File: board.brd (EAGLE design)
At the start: 25.3 x 23.8 mm, 30 parts, among them U3 ATTINY1607-MFR, U4 RV-8803, X2 JST_SM02B-SRSS-TB

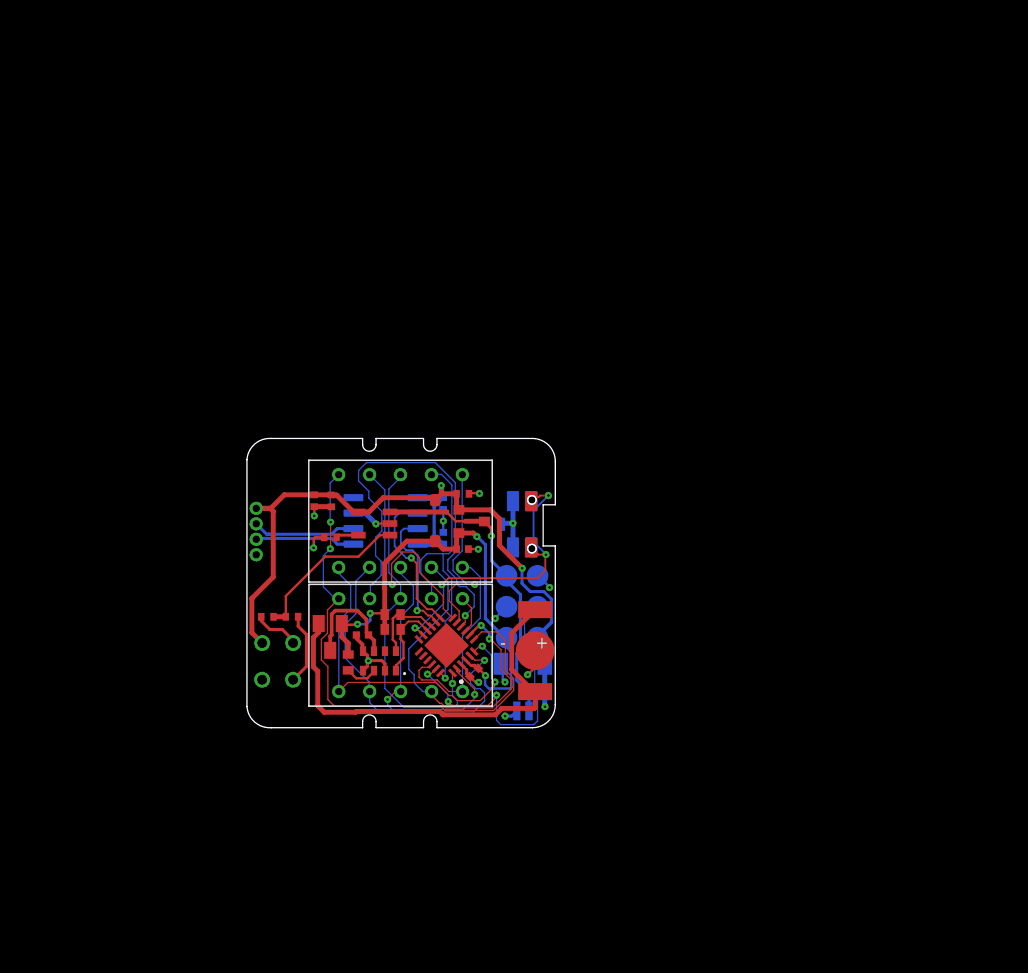
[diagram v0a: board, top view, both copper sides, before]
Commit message: added next dev board
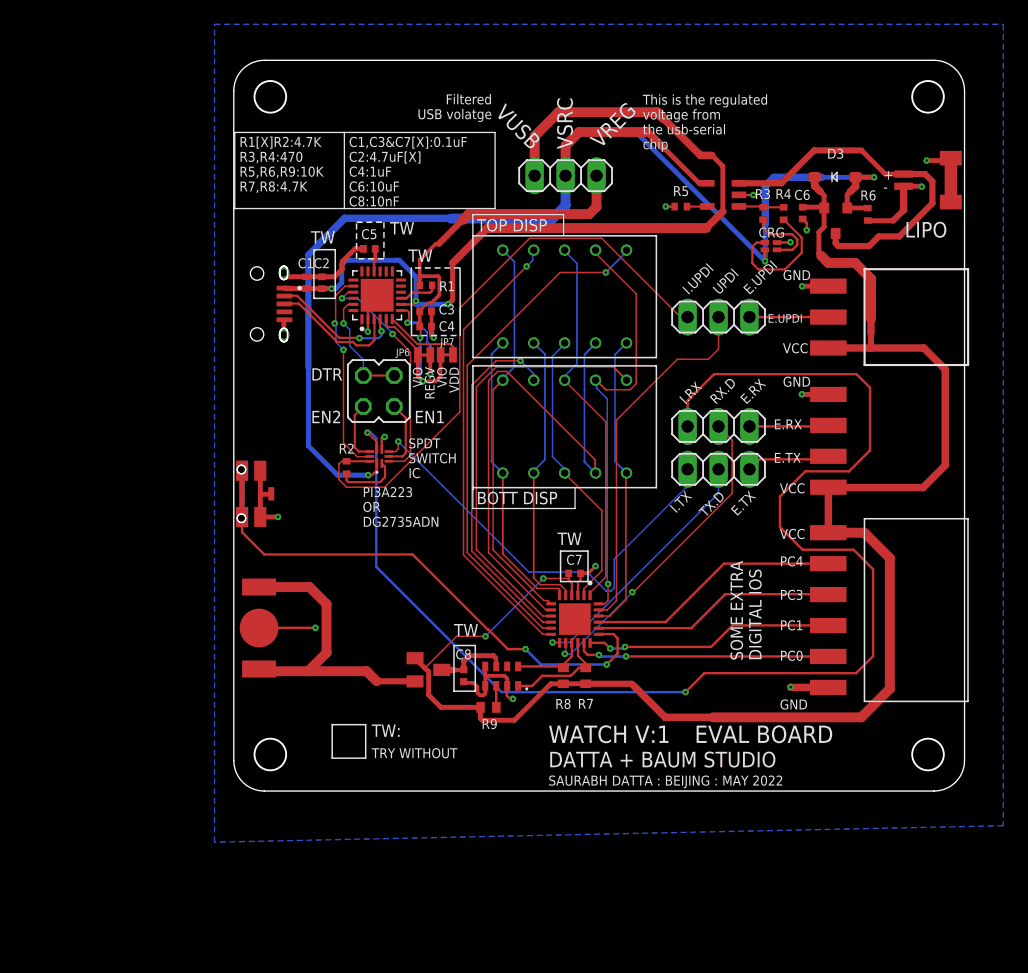
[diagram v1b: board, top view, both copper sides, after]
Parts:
- removed D2: BAS70-05, BAS_40_05:SOT23
- removed GREEN: GREEN, MY_CLOCK_LIB_COMPONENTS:2MMLED_GREEN
- removed U$3: DMG341, MY_CLOCK_LIB_COMPONENTS:DMG341-P_CHANNEL_MOSFET-SOT23
- removed U$4: PTS840ESDPMSMTRLF, MY_CLOCK_LIB_COMPONENTS:PTS840ESDPMSMTRLF
- removed U$5: 4X1.27_FEMALE_EMPTY_CONN, MY_CLOCK_LIB_COMPONENTS:4X1.27_FEMALE_EMPTY_CONN-BACKUP
- removed U$6: CH330N, MY_CLOCK_LIB_COMPONENTS:CH330N
- removed YELLOW: ORANGE, MY_CLOCK_LIB_COMPONENTS:2MMLED_YELLOW
- added 2IN1LED: HSMF-C16, MY_CONNECTORS:HSMF-C16
- added C8: 10nF, SparkFun-Capacitors:0402-TIGHT
- added D3: MBR0540, Diodes:SOD-123
- added J1: 1x4 RA Female, MY_CLOCK_LIB_COMPONENTS:1X04_SMD_RA_FEMALE
- added J2: 1x3 RA Female, SparkFun-Connectors:1X03_SMD_RA_FEMALE
- added J3: (no value), SparkFun-Connectors:1X06-SMD-FEMALE
- added JP1: 2X2PIN_JUMPER, MY_CONNECTORS:2X2PIN_JUMPER
- added JP2, JP3, JP4, JP5: PINHD-1X3, Connector:1X03
- added JP6, JP7: JUMPER-SMT_2_NC_TRACE_NO-SILK, SparkFun-Jumpers:SMT-JUMPER_2_NC_TRACE_NO-SILK
- added R8, R9: 4.7K, ARDUINO_3V_TTL_INTERFACE_2_PI:ADAFRUIT_R0402
- added U$10: MCP, MY_CLOCK_LIB_COMPONENTS:MCP73831_SOT23-5L
- added U$11: DMG341, MY_CLOCK_LIB_COMPONENTS:DMG341-P_CHANNEL_MOSFET-SOT23
- added U$8: VERTICAL_MICRO_USBCUI_HOR_T4, MY_CLOCK_LIB_COMPONENTS:CUI_UJ2-MIBH-4-SMT-TR-67
- added U2: CP2104-F03-GM, CP2104-F03-GM:QFN50P400X400X80-25N
- C3: value 100nF -> 0.1uF
- C4: value 10uF -> 1uF
- C5: value 100nF -> 4.7uF
- C6: value 10nF -> 10uF; device SparkFun-Capacitors:0402-TIGHT -> MY_CAP_LIB:CAPC1005X60
- D1: value MBR0540 -> BAS70-05; device Diodes:SOD-123 -> BAS_40_05:SOT23
- R1, R2: value 470 -> 4.7K
- R3: value 10K -> 470
- R4: value 4.7K -> 470; device ARDUINO_3V_TTL_INTERFACE_2_PI:ADAFRUIT_R0402 -> resistor:RESC1005X40
- R5: value 4.7K -> 10K; device ARDUINO_3V_TTL_INTERFACE_2_PI:ADAFRUIT_R0402 -> resistor:RESC1005X40
- U$1: value MCP73831/2_LIPO_CHARGER -> PI3A223; device MY_CLOCK_LIB_COMPONENTS:MCP73831_SOT23-5L -> MY_CLOCK_LIB_COMPONENTS:QFN40P140X180X60-10N
- U$2: value 2X3_PAD_ARRAY -> PTS840ESDPMSMTRLF; device MY_CLOCK_LIB_COMPONENTS:2X3_PAD_ARRAY -> MY_CLOCK_LIB_COMPONENTS:PTS840ESDPMSMTRLF
- moved X2 53.6 mm to (54.7, 45.7), flipped to the top, turned to 270 degrees
- moved C6 50.1 mm to (46.4, 43.0), turned to 270 degrees
- moved R4 46.9 mm to (44.8, 43.0), turned to 90 degrees
- moved R3 44.4 mm to (43.1, 43.0), turned to 90 degrees
- moved R5 41.0 mm to (36.4, 43.5), turned to 180 degrees
- moved R6 40.4 mm to (51.7, 42.9), turned to 90 degrees
- moved R1 30.2 mm to (15.4, 37.1)
- moved TOP 22.8 mm to (26.8, 36.1)
- moved 1.55V-8MAH 22.7 mm to (1.75, 8.94), turned to 90 degrees
- moved BOT 22.4 mm to (26.8, 25.5)
- moved U$2 22.0 mm to (1.10, 19.9), flipped to the top
- moved C5 21.8 mm to (10.8, 40.1), flipped to the top, turned to 180 degrees
- moved R7 19.5 mm to (28.6, 5.01), turned to 90 degrees
- moved C3 18.7 mm to (15.4, 35.0), flipped to the top, turned to 180 degrees
- moved C4 18.5 mm to (15.4, 33.7), turned to 180 degrees
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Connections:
- removed net USBD_N: U$5.USBD_N, U$6.D_N
- removed net USBD_P: U$5.USBD_P, U$6.D_P
- new net !RST: R1.2, U2.9
- new net DTR: JP1.1, JP1.3, U2.23
- new net IN1: JP1.2, U$1.IN1
- new net IN2: JP1.4, U$1.IN2
- new net NO1: R2.2, U$1.NO1
- new net PC0: J3.5, U3.17
- new net PC1: J3.4, U3.18
- new net PC3: J3.3, U3.20
- new net PC4: J3.2, U3.21
- new net REGIN: JP6.2, U2.7
- new net RX_AS: JP5.3, U$1.NC2
- new net RX_CP: U$1.COM2, U2.20
- new net RX_EXT: J1.3, JP5.1
- new net TX_AS: JP4.3, U$1.NC1
- new net TX_CP: U$1.COM1, U2.21
- new net TX_EXT: J1.2, JP4.1
- new net UPDI_EXT: J2.2, JP3.1
- new net UPDI_INT: JP3.3, R2.1, U$1.NO2
- new net USB_N: U$8.2, U2.4
- new net USB_P: U$8.3, U2.3
- new net VBUS: C1.1, C2.1, JP2.1, U$8.1, U2.8
- new net VDD: JP7.1, U2.6
- new net VIO: C3.2, C4.2, JP2.3, JP6.1, JP7.2, R1.1, U2.5
- new net VPP: C5.1, U2.16
- net !INT: now also R9.2; no longer R7.2
- net CHARGER_PROG: now also R5.1, U$10.5; no longer R3.1, U$1.5
- net CHARGER_STAT: now also R3.2, R4.2, U$10.1; no longer R1.2, R2.2, U$1.1
- net GND: now also 2IN1LED.P$3, C3.1, C4.1, C8.2, J1.4, J2.3, J3.6, R5.2, U$1.GND, U$10.2, U$2.1, U$2.5, U$8.5, U$8.S1, U$8.S2, U2.2, U2.25; no longer C3.2, C4.2, GREEN.K, R3.2, U$1.2, U$2.6, U$4.1, U$4.2, U$4.5, U$5.GND, U$6.GND
- net LEDG_A: now also 2IN1LED.P$1, R4.1; no longer GREEN.A, R2.1
- net LEDY_K: now also 2IN1LED.P$4, R3.1; no longer R1.1, YELLOW.K
- net RX: now also JP5.2; no longer U$6.RXI
- net SCL: now also R7.2; no longer R4.2
- net SDA: now also R8.2; no longer R5.2
- net SW1: now also U$2.3, U$2.4, U$2.B3, U$2.B4, U3.19; no longer U$4.3, U$4.4, U$4.B3, U$4.B4, U3.17
- net TX: now also JP4.2; no longer U$6.TXD
- net UPDI: now also JP3.2; no longer U$2.5
- net VBATT: now also D1.2; no longer D2.2
- net VCC: now also C6.1, D1.1, D3.C, J1.1, J2.1, J3.1, R8.1, R9.1, U$11.2; no longer C4.1, D1.C, D2.1, R4.1, R5.1, U$2.3, U$3.2
- net VDD1: now also C8.1, D1.3; no longer C6.1, D2.3
- net V_LIPO: now also U$10.3, U$11.3; no longer U$1.3, U$2.1, U$3.3
- net V_USB: now also 2IN1LED.P$2, D3.A, JP2.2, U$1.VDD, U$10.4, U$11.1; no longer C1.1, C2.1, C3.1, C5.1, D1.A, U$1.4, U$2.4, U$3.1, U$5.V_USB, U$6.V3, U$6.VCC, YELLOW.A
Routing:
- net RX_AS: track 0.00 -> 110.7 mm, vias 0 -> 2
- net VCC: track 41.4 -> 131.2 mm, vias 4 -> 2
- net VBUS: track 0.00 -> 72.1 mm, vias 0 -> 3
- net V_USB: track 60.7 -> 110.7 mm, vias 2 -> 3
- net UPDI_INT: track 0.00 -> 48.9 mm
- net VIO: track 0.00 -> 42.3 mm, vias 0 -> 2
- net TX_AS: track 0.00 -> 36.6 mm, vias 0 -> 1
- net COMM4: track 3.13 -> 35.2 mm
- net GND: track 35.5 -> 63.3 mm, vias 15 -> 16
- net COMM2: track 15.7 -> 41.9 mm
- net SW1: track 25.1 -> 47.5 mm, vias 4 -> 2
- net PC0: track 0.00 -> 20.9 mm, vias 0 -> 2
- net PC4: track 0.00 -> 20.8 mm
- net PC1: track 0.00 -> 20.5 mm, vias 0 -> 2
- net PC3: track 0.00 -> 20.0 mm
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- added copper zone on layer 16, net GND
- removed copper zone on layer 15, net GND
- removed copper zone on layer 2, net GND
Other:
- board size 25.3 x 23.8 mm -> 60 x 60 mm
- board text added: "BOTT DISP"
- board text added: "C1,C3&C7[X]:0.1uF C2:4.7uF[X] C4:1uF C6:10uF C8:10nF"
- board text added: "CRG"
- board text added: "DATTA + BAUM STUDIO"
- board text added: "DTR"
- board text added: "E.RX"
- board text added: "E.TX"
- board text added: "E.UPDI"
- board text added: "EN1"
- board text added: "EN2"
- board text added: "EVAL BOARD"
- board text added: "Filtered USB volatge"
- board text added: "GND"
- board text added: "I.RX"
- board text added: "I.TX"
- board text added: "I.UPDI"
- board text added: "LIPO"
- board text added: "PC0"
- board text added: "PC1"
- board text added: "PC3"
- board text added: "PC4"
- board text added: "PI3A223 OR DG2735ADN"
- board text added: "R1[X]R2:4.7K R3,R4:470 R5,R6,R9:10K R7,R8:4.7K"
- board text added: "REGV"
- board text added: "RX.D"
- board text added: "SAURABH DATTA : BEIJING : MAY 2022"
- board text added: "SOME EXTRA DIGITAL IOS"
- board text added: "SPDT SWITCH IC"
- board text added: "TOP DISP"
- board text added: "TRY WITHOUT"
- board text added: "TW"
- board text added: "TW:"
- board text added: "TX.D"
- board text added: "This is the regulated voltage from the usb-serial chip"
- board text added: "UPDI"
- board text added: "VCC"
- board text added: "VDD"
- board text added: "VIO"
- board text added: "VREG"
- board text added: "VSRC"
- board text added: "VUSB"
- board text added: "WATCH V:1"
- board text removed: "P1"
- board text removed: "P2"
- board text removed: "P3"
- board text removed: "P4"
- board text removed: "P5"
- board text removed: "P6"

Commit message: first commit
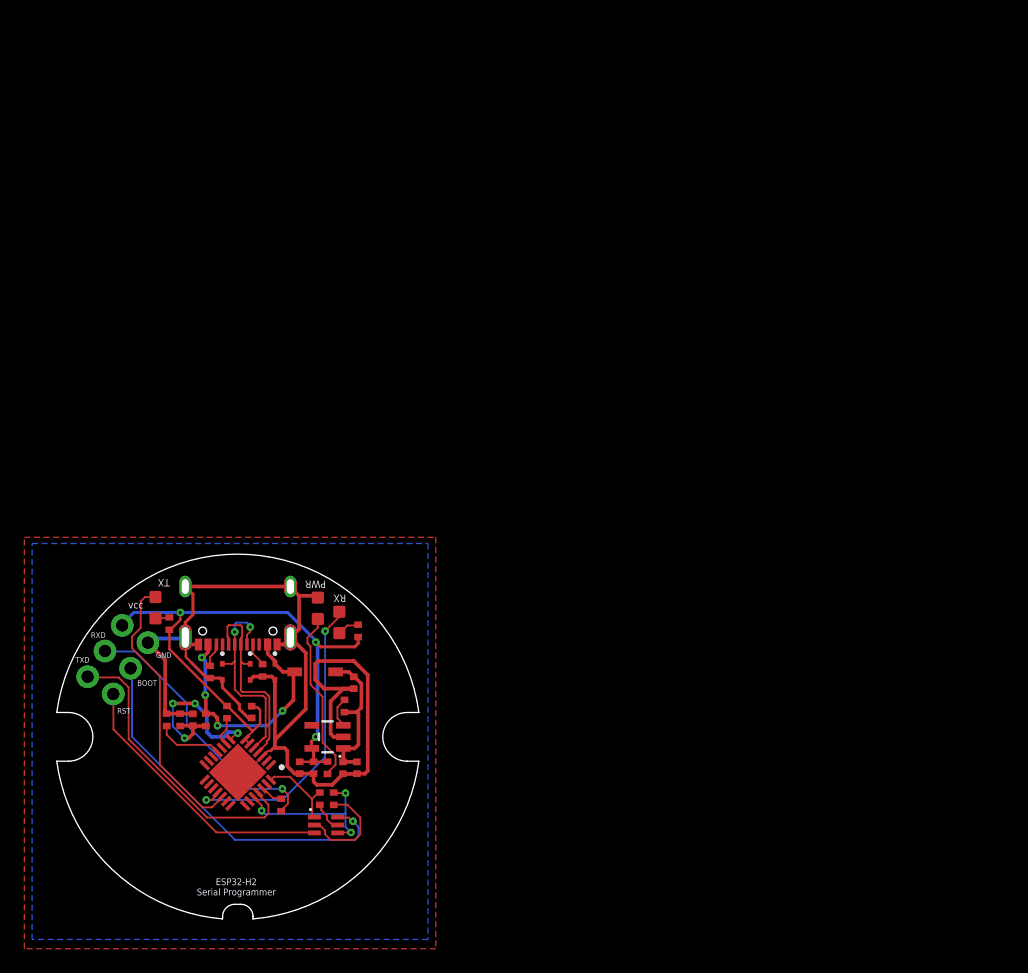
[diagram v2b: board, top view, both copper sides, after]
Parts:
- removed 1.55V-8MAH: BK-414-TR, MY_CLOCK_LIB_COMPONENTS:BK-414-TR
- removed 2IN1LED: HSMF-C16, MY_CONNECTORS:HSMF-C16
- removed BOT, TOP: 0.28-2DIGIT-7SEGEMNT, MY_CLOCK_LIB_COMPONENTS:2_DIGIT_0.28
- removed C8: 10nF, SparkFun-Capacitors:0402-TIGHT
- removed J3: (no value), SparkFun-Connectors:1X06-SMD-FEMALE
- removed JP1: 2X2PIN_JUMPER, MY_CONNECTORS:2X2PIN_JUMPER
- removed JP2, JP3, JP4, JP5: PINHD-1X3, Connector:1X03
- removed JP6, JP7: JUMPER-SMT_2_NC_TRACE_NO-SILK, SparkFun-Jumpers:SMT-JUMPER_2_NC_TRACE_NO-SILK
- removed U$1: PI3A223, MY_CLOCK_LIB_COMPONENTS:QFN40P140X180X60-10N
- removed U$10: MCP, MY_CLOCK_LIB_COMPONENTS:MCP73831_SOT23-5L
- removed U$11: DMG341, MY_CLOCK_LIB_COMPONENTS:DMG341-P_CHANNEL_MOSFET-SOT23
- removed U$2: PTS840ESDPMSMTRLF, MY_CLOCK_LIB_COMPONENTS:PTS840ESDPMSMTRLF
- removed U$8: VERTICAL_MICRO_USBCUI_HOR_T4, MY_CLOCK_LIB_COMPONENTS:CUI_UJ2-MIBH-4-SMT-TR-67
- removed U2: CP2104-F03-GM, CP2104-F03-GM:QFN50P400X400X80-25N
- removed U3: ATTINY1607-MFR, ATTINY1607-MNR:QFN50P400X400X90-25N
- removed U4: RV-8803, RV-8803:RV-3028
- removed X2: JST_SM02B-SRSS-TB, MY_CLOCK_LIB_COMPONENTS:JST-SM02B-SRSS-TB
- added AP2112_3.3V: 3.3V, Help-by-jennyfer-button-design-lib:SOT23-5
- added D2, D4: D5V0L1B2LP4-7B, Help-by-jennyfer-button-design-lib:D5V0L1B2LP4-7B
- added IC1: CP2102N-A02-GQFN28, Help-by-jennyfer-button-design-lib:QFN50P500X500X80-29N
- added IC2: BC847BDW1T1G (DUAL NPN), Help-by-jennyfer-button-design-lib:SOT65P210X110-6N
- added R10, R12, R13: 10K, Help-by-jennyfer-button-design-lib:RESC1005X40
- added R11: 5.1K, Help-by-jennyfer-button-design-lib:RESC1005X40
- added RX_LED, TX_LED, USB_POWER_LED: GREEN, Help-by-jennyfer-button-design-lib:LED-0603
- C1, C7: value 100nF -> 10uF; device MY_CAP_LIB:CAPC1005X60 -> Help-by-jennyfer-button-design-lib:CAPC1005X60
- C2: value 4.7uF -> 10uF; device MY_CAP_LIB:CAPC1005X60 -> Help-by-jennyfer-button-design-lib:CAPC1005X60
- C3: value 0.1uF -> 1uF; device MY_CAP_LIB:CAPC1005X60 -> Help-by-jennyfer-button-design-lib:CAPC1005X60
- C4: value 1uF -> 10uF; device MY_CAP_LIB:CAPC1005X60 -> Help-by-jennyfer-button-design-lib:CAPC1005X60
- C5: value 4.7uF -> 0.1uF; device MY_CAP_LIB:CAPC1005X60 -> Help-by-jennyfer-button-design-lib:CAPC1005X60
- C6: value 10uF -> 0.1uF; device MY_CAP_LIB:CAPC1005X60 -> Help-by-jennyfer-button-design-lib:CAPC1005X60
- D1: value BAS70-05 -> 1N5819HW-7-F; device BAS_40_05:SOT23 -> Help-by-jennyfer-button-design-lib:SOD3715X145N
- D3: value MBR0540 -> D5V0L1B2LP4-7B; device Diodes:SOD-123 -> Help-by-jennyfer-button-design-lib:D5V0L1B2LP4-7B
- J1: value 1x4 RA Female -> (none); device MY_CLOCK_LIB_COMPONENTS:1X04_SMD_RA_FEMALE -> Help-by-jennyfer-button-design-lib:USB-C-16P-2LAYER-PADS
- J2: value 1x3 RA Female -> 2X3_2.5_prog; device SparkFun-Connectors:1X03_SMD_RA_FEMALE -> Help-by-jennyfer-button-design-lib:2X3_PROG_POGOS
- R1, R2: value 4.7K -> 5.1K; device resistor:RESC1005X40 -> Help-by-jennyfer-button-design-lib:RESC1005X40
- R3: value 470 -> 22.1K; device resistor:RESC1005X40 -> Help-by-jennyfer-button-design-lib:RESC1005X40
- R4: value 470 -> 47.5K; device resistor:RESC1005X40 -> Help-by-jennyfer-button-design-lib:RESC1005X40
- R5: value 10K -> 1K; device resistor:RESC1005X40 -> Help-by-jennyfer-button-design-lib:RESC1005X40
- R6: device resistor:RESC1005X40 -> Help-by-jennyfer-button-design-lib:RESC1005X40
- R7, R8: value 4.7K -> 100; device ARDUINO_3V_TTL_INTERFACE_2_PI:ADAFRUIT_R0402 -> Help-by-jennyfer-button-design-lib:RESC1005X40
- R9: value 4.7K -> 470; device ARDUINO_3V_TTL_INTERFACE_2_PI:ADAFRUIT_R0402 -> Help-by-jennyfer-button-design-lib:RESC1005X40
- moved R6 71.0 mm to (-5.84, 1.40)
- moved J2 69.9 mm to (-9.49, 9.15), turned to 236 degrees
- moved R4 64.7 mm to (-4.74, 1.40), turned to 270 degrees
- moved D3 64.7 mm to (-1.27, 5.33), turned to 270 degrees
- moved R3 61.8 mm to (-2.62, 1.40), turned to 270 degrees
- moved C6 60.7 mm to (6.22, -2.53)
- moved J1 58.3 mm to (0.00, 7.24), turned to 180 degrees
- moved R5 55.8 mm to (-0.89, 2.03), turned to 90 degrees
- moved C5 42.6 mm to (9.78, -2.54), turned to 270 degrees
- moved C3 38.6 mm to (-3.68, 1.40), turned to 90 degrees
- moved C4 36.9 mm to (8.64, -2.54), turned to 270 degrees
- moved R1 36.4 mm to (-2.29, 5.33), turned to 90 degrees
- moved C2 35.7 mm to (1.14, 2.03), turned to 270 degrees
- moved R7 34.5 mm to (-5.63, 9.30), turned to 270 degrees
- moved C1 33.1 mm to (9.53, 4.45), turned to 270 degrees
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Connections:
- removed net !INT: R9.2, U4.6
- removed net !RST: R1.2, U2.9
- removed net CHARGER_PROG: R5.1, U$10.5
- removed net CHARGER_STAT: R3.2, R4.2, U$10.1
- removed net COMM1: TOP._9, U3.12
- removed net COMM2: TOP._6, U3.11
- removed net COMM3: BOT._9, U3.10
- removed net COMM4: BOT._6, U3.9
- removed net DOT: BOT._5, TOP._5, U3.22
- removed net IN1: JP1.2, U$1.IN1
- removed net IN2: JP1.4, U$1.IN2
- removed net LEDG_A: 2IN1LED.P$1, R4.1
- removed net LEDY_K: 2IN1LED.P$4, R3.1
- removed net NO1: R2.2, U$1.NO1
- removed net PC0: J3.5, U3.17
- removed net PC1: J3.4, U3.18
- removed net PC3: J3.3, U3.20
- removed net PC4: J3.2, U3.21
- removed net REGIN: JP6.2, U2.7
- removed net RX: JP5.2, U3.14
- removed net RX_AS: JP5.3, U$1.NC2
- removed net RX_CP: U$1.COM2, U2.20
- removed net RX_EXT: J1.3, JP5.1
- removed net SCL: R7.2, U3.16, U4.8
- removed net SDA: R8.2, U3.15, U4.1
- removed net SEG_A: BOT._7, TOP._7, U3.24
- removed net SEG_B: BOT._8, TOP._8, U3.1
- removed net SEG_C: BOT._3, TOP._3, U3.2
- removed net SEG_D: BOT._2, TOP._2, U3.5
- removed net SEG_E: BOT._1, TOP._1, U3.6
- removed net SEG_F: BOT._10, TOP._10, U3.7
- removed net SEG_G: BOT._4, TOP._4, U3.8
- removed net SW1: U$2.3, U$2.4, U$2.B3, U$2.B4, U3.19
- removed net TX: JP4.2, U3.13
- removed net TX_AS: JP4.3, U$1.NC1
- removed net TX_CP: U$1.COM1, U2.21
- removed net TX_EXT: J1.2, JP4.1
- removed net UPDI: JP3.2, U3.23
- removed net UPDI_EXT: J2.2, JP3.1
- removed net UPDI_INT: JP3.3, R2.1, U$1.NO2
- removed net USB_N: U$8.2, U2.4
- removed net USB_P: U$8.3, U2.3
- removed net VBATT: 1.55V-8MAH.1+, 1.55V-8MAH.2+, D1.2
- removed net VCC: C6.1, C7.1, D1.1, D3.C, J1.1, J2.1, J3.1, R7.1, R8.1, R9.1, U$11.2, U3.4
- removed net VDD: JP7.1, U2.6
- removed net VDD1: C8.1, D1.3, U4.3
- removed net VIO: C3.2, C4.2, JP2.3, JP6.1, JP7.2, R1.1, U2.5
- removed net VPP: C5.1, U2.16
- removed net V_LIPO: U$10.3, U$11.3, X2.2
- removed net V_USB: 2IN1LED.P$2, D3.A, JP2.2, R6.2, U$1.VDD, U$10.4, U$11.1
- new net CHIP_PU/RST/EN: IC2.3, J2.6
- new net GPIO_9/BOOT: IC2.6, J2.4
- new net N$10: R11.2, USB_POWER_LED.A
- new net N$11: IC2.2, R12.1
- new net N$12: IC2.5, R13.2
- new net N$2: J1.B5, R1.2
- new net N$3: R7.1, TX_LED.A
- new net N$4: J1.A5, R2.2
- new net N$5: R8.1, RX_LED.A
- new net RSTB: IC1.9, R5.1
- new net RTS: IC1.24, IC2.4, R12.2
- new net RXT: IC1.18, RX_LED.C
- new net SUSPENDDB: IC1.11, R6.1
- new net TXD: IC1.26, R9.1
- new net TXT: IC1.19, TX_LED.C
- new net UART_RXD: J2.3, R9.2
- new net UART_TXD: IC1.25, J2.5
- new net USB_D_N: D3.1, IC1.5, J1.A7, J1.B7
- new net USB_D_P: D4.1, IC1.4, J1.A6, J1.B6
- new net VBUSA: D1.2, D2.1, J1.VBUS1, J1.VBUS2, R3.1
- new net VCC_3V3: AP2112_3.3V.5, C2.1, C6.1, C7.1, IC1.6, IC1.7, J2.1, R11.1, R5.2, R7.2, R8.2
- new net VCC_5V: AP2112_3.3V.1, C1.1, C4.1, C5.1, D1.1, R10.1
- new net VREG_EN: AP2112_3.3V.3, R10.2
- net DTR: now also IC1.28, IC2.1, R13.1; no longer JP1.1, JP1.3, U2.23
- net GND: now also AP2112_3.3V.2, C3.2, C4.2, D2.2, D3.2, D4.2, IC1.29, IC1.3, J1.GND, J1.GND2, J1.SHLD1, J1.SHLD2, J1.SHLD3, J1.SHLD4, J2.2, R1.1, R2.1, R4.1, R6.2, USB_POWER_LED.C; no longer 1.55V-8MAH.-, 2IN1LED.P$3, C3.1, C4.1, C8.2, J1.4, J2.3, J3.6, R5.2, R6.1, U$1.GND, U$10.2, U$2.1, U$2.2, U$2.5, U$8.5, U$8.S1, U$8.S2, U2.2, U2.25, U3.3, U4.4, U4.5, U4.7, X2.1, X2.M1, X2.M2
- net VBUS: now also C3.1, IC1.8, R3.2, R4.2; no longer C1.1, C2.1, JP2.1, U$8.1, U2.8
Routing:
- net VCC: track 131.2 -> 0.00 mm, vias 2 -> 0
- net RX_AS: track 110.7 -> 0.00 mm, vias 2 -> 0
- net V_USB: track 110.7 -> 0.00 mm, vias 3 -> 0
- net VBUS: track 72.1 -> 15.2 mm, vias 3 -> 4
- net VCC_3V3: track 0.00 -> 51.7 mm, vias 0 -> 3
- net UPDI_INT: track 48.9 -> 0.00 mm
- net SW1: track 47.5 -> 0.00 mm, vias 2 -> 0
- net SEG_G: track 45.8 -> 0.00 mm
- net VIO: track 42.3 -> 0.00 mm, vias 2 -> 0
- net COMM2: track 41.9 -> 0.00 mm, vias 1 -> 0
- net COMM1: track 37.3 -> 0.00 mm, vias 1 -> 0
- net GND: track 63.3 -> 99.9 mm, vias 16 -> 0
- net TX_AS: track 36.6 -> 0.00 mm, vias 1 -> 0
- net SEG_A: track 35.6 -> 0.00 mm, vias 1 -> 0
- net COMM4: track 35.2 -> 0.00 mm
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- added copper zone on layer 1, net GND
- added copper zone on layer 16, net VCC_3V3
- removed copper zone on layer 16, net GND
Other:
- board size 60 x 60 mm -> 29.7 x 29.9 mm
- board text added: ""HELP" by"
- board text added: "BOOT"
- board text added: "ESP32-H2 Serial Programmer"
- board text added: "PWR"
- board text added: "RST"
- board text added: "RX"
- board text added: "RXD"
- board text added: "TX"
- board text added: "TXD"
- board text added: "vcc"
- board text removed: "+"
- board text removed: "-"
- board text removed: "BOTT DISP"
- board text removed: "C1,C3&C7[X]:0.1uF C2:4.7uF[X] C4:1uF C6:10uF C8:10nF"
- board text removed: "CRG"
- board text removed: "DATTA + BAUM STUDIO"
- board text removed: "DTR"
- board text removed: "E.RX"
- board text removed: "E.TX"
- board text removed: "E.UPDI"
- board text removed: "EN1"
- board text removed: "EN2"
- board text removed: "EVAL BOARD"
- board text removed: "Filtered USB volatge"
- board text removed: "I.RX"
- board text removed: "I.TX"
- board text removed: "I.UPDI"
- board text removed: "LIPO"
- board text removed: "PC0"
- board text removed: "PC1"
- board text removed: "PC3"
- board text removed: "PC4"
- board text removed: "PI3A223 OR DG2735ADN"
- board text removed: "R1[X]R2:4.7K R3,R4:470 R5,R6,R9:10K R7,R8:4.7K"
- board text removed: "REGV"
- board text removed: "RX.D"
- board text removed: "SAURABH DATTA : BEIJING : MAY 2022"
- board text removed: "SOME EXTRA DIGITAL IOS"
- board text removed: "SPDT SWITCH IC"
- board text removed: "TOP DISP"
- board text removed: "TRY WITHOUT"
- board text removed: "TW"
- board text removed: "TW:"
- board text removed: "TX.D"
- board text removed: "This is the regulated voltage from the usb-serial chip"
- board text removed: "UPDI"
- board text removed: "VCC"
- board text removed: "VDD"
- board text removed: "VIO"
- board text removed: "VREG"
- board text removed: "VSRC"
- board text removed: "VUSB"
- board text removed: "WATCH V:1"
